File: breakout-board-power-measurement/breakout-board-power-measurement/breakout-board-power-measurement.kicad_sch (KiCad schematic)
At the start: 61 parts, among them J1 Screw_Terminal_01x04, J2 Conn_01x07, J3 Conn_01x07, J4 Conn_01x02, Q1 NMOS, Q2 NMOS, U1 MCP3911A0-E/SS, U2 Si8641BA-B-IU, U3 LM317_3PinPackage, Y1 10M

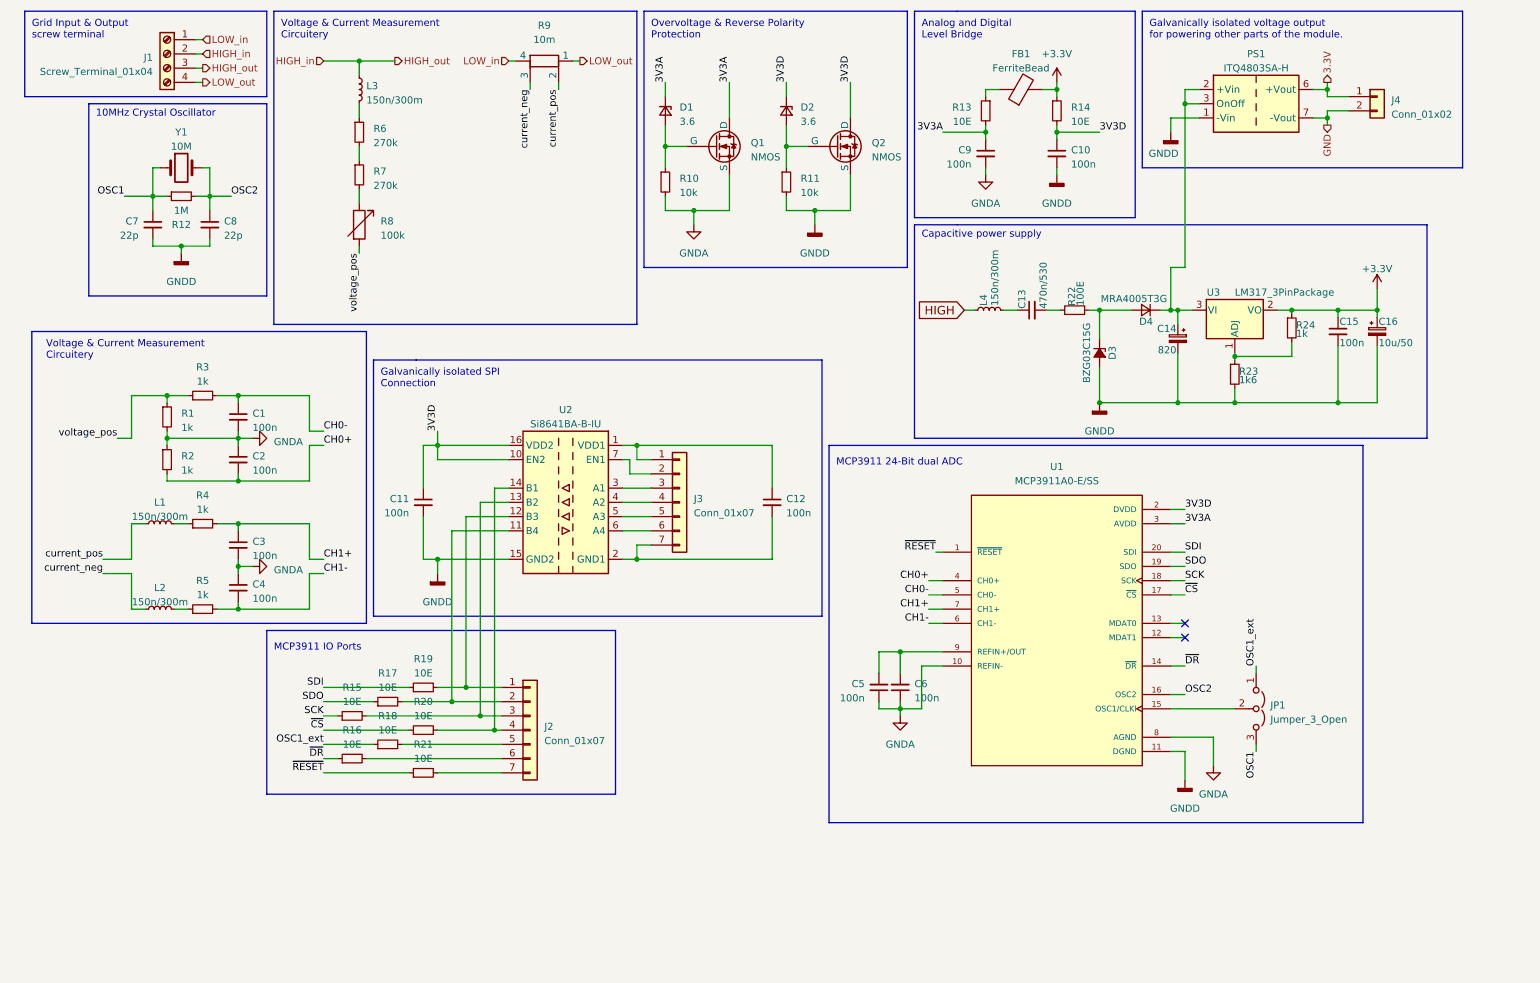
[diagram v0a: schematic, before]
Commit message: Major updates: Power Measurement PCB-routing half way done.
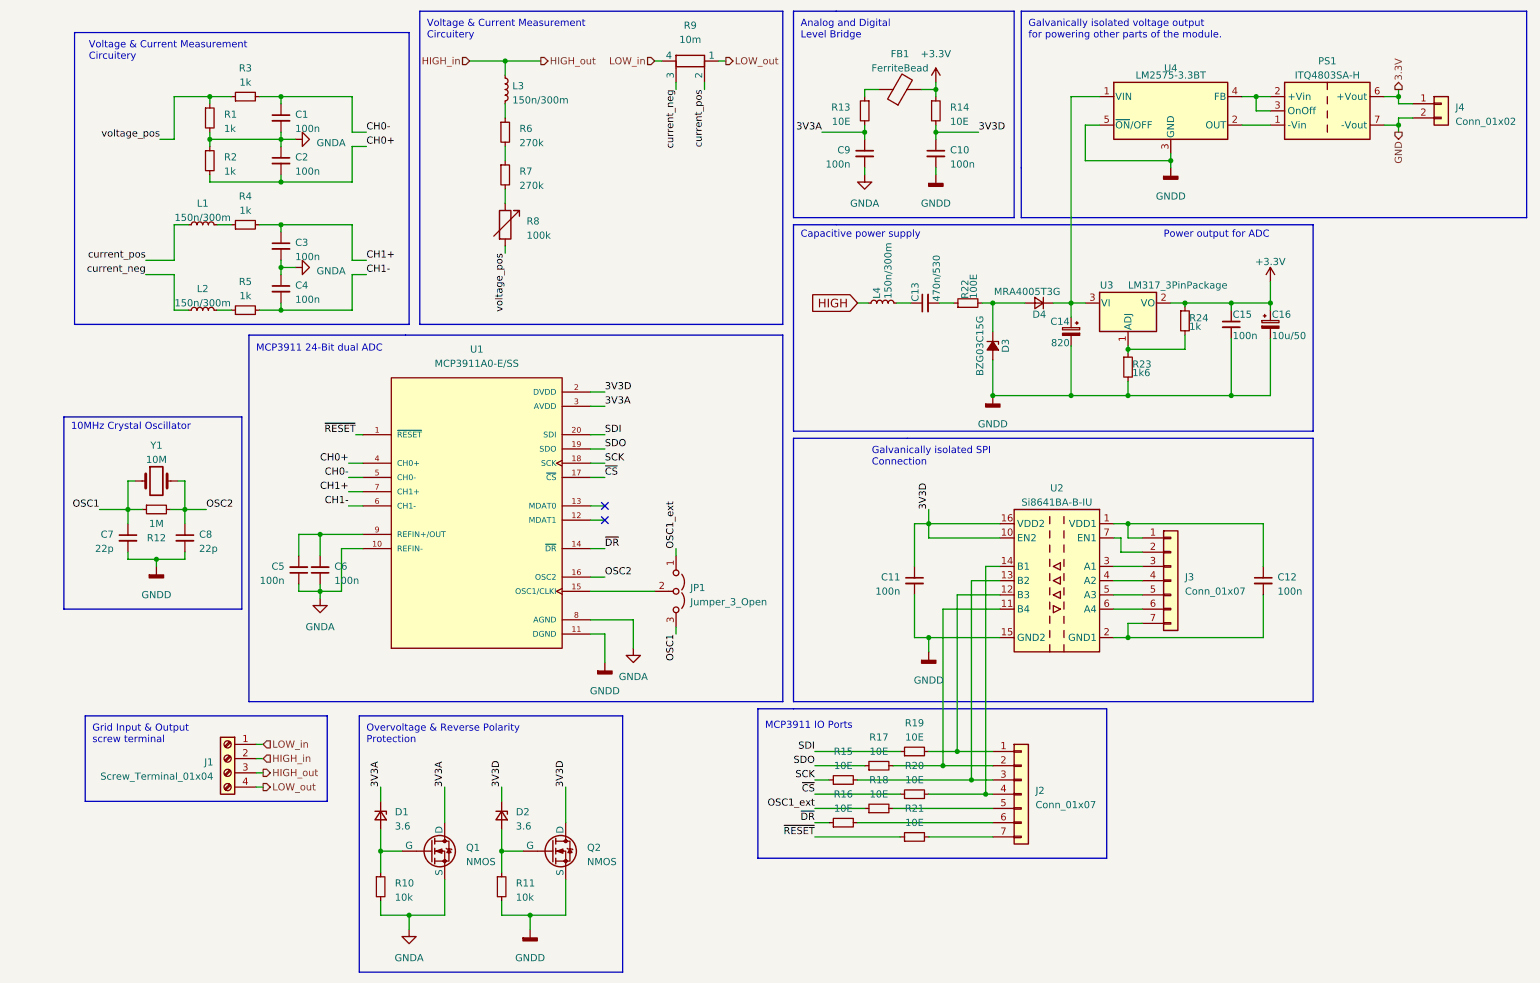
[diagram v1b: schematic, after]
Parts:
- added U4: LM2575-3.3BT, Package_TO_SOT_THT:TO-220-5_Vertical, symbol Regulator_Switching:LM2575-3.3BT
- JP1: footprint (none) -> Pin_Headers:Pin_Header_Straight_1x03_Pitch2.54mm
- L1, L2, L3: footprint (none) -> Inductors_SMD:L_1206_HandSoldering
- R9: footprint (none) -> Resistors_THT:R_Axial_DIN0516_L15.5mm_D5.0mm_P20.32mm_Horizontal
- U1: footprint (none) -> Housings_SSOP:SSOP-20_5.3x7.2mm_Pitch0.65mm
- Y1: footprint (none) -> Crystals:Crystal_HC49-4H_Vertical
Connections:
- net GNDD: now also U4.3 (GND), U4.5 (~{ON}/OFF); no longer PS1.1 (-Vin)
- net at C14.1, D4.1 (K), U3.3 (VI): now also U4.1 (VIN); no longer PS1.2 (+Vin), PS1.3 (OnOff)
- new net: PS1.1 (-Vin), U4.2 (OUT)
- new net: PS1.2 (+Vin), PS1.3 (OnOff), U4.4 (FB)
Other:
- note added: "Power output for ADC"
- moved on the sheet: C1, C10, C11, C12, C13, C14, C15, C16, C2, C3, C4, C5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
